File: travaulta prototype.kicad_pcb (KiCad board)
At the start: 4 copper layers, 209.7 x 76.4 mm, 106 parts, among them SW1 EC_SW, SW10 EC_SW, SW11 EC_SW, SW12 EC_SW, SW13 EC_SW, SW14 EC_SW, SW15 EC_SW, SW16 EC_SW, SW17 EC_SW, SW18 EC_SW, SW19 EC_SW, SW2 EC_SW, SW20 EC_SW, SW21 EC_SW, SW22 EC_SW, SW23 EC_SW, SW24 EC_SW, SW25 EC_SW, SW26 EC_SW, SW27 EC_SW, SW28 EC_SW, SW29 EC_SW, SW3 EC_SW, SW30 EC_SW, SW31 EC_SW, SW32 EC_SW, SW33 EC_SW, SW34 EC_SW, SW35 EC_SW, SW36 EC_SW, SW37 EC_SW, SW38 BOOT0, SW4 EC_SW, SW5 EC_SW, SW6 EC_SW, SW7 EC_SW, SW8 EC_SW, SW9 EC_SW, U1 STM32F401CBUx, U2 XC6206PxxxMR, U3 74HC4051, U4 74HC4051, U5 OPA350, Y1 8 MHz

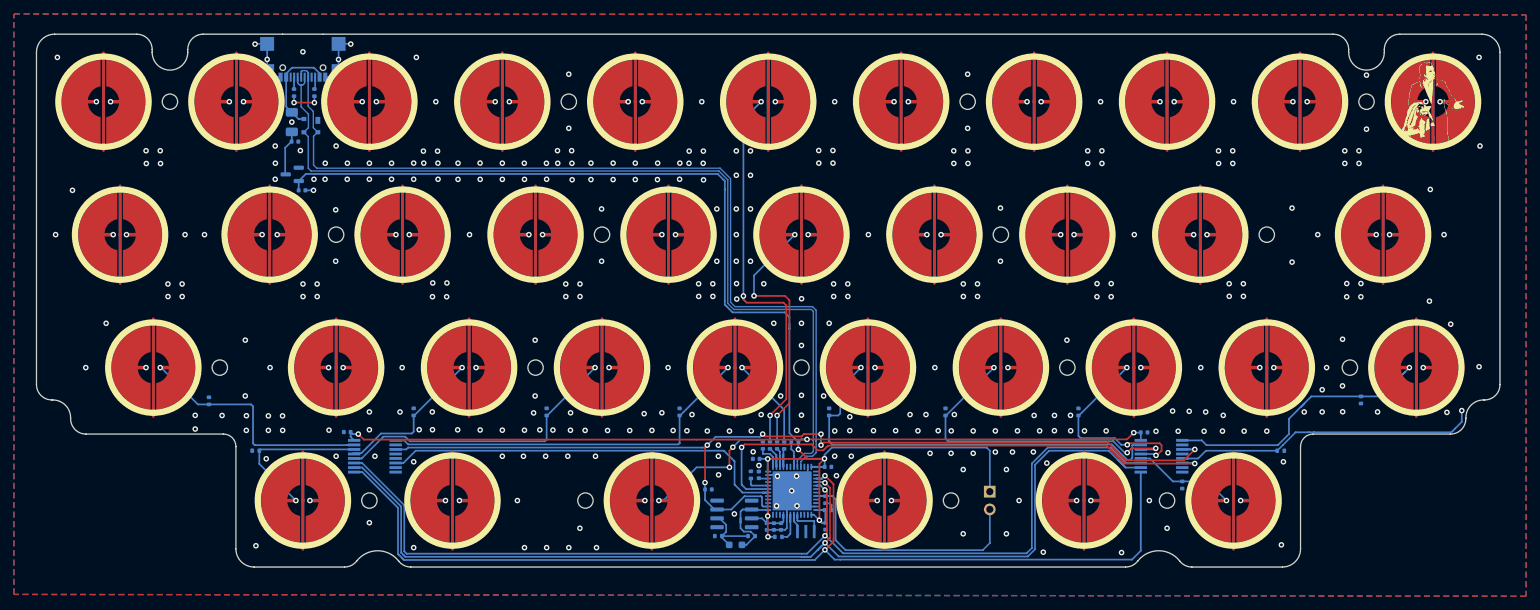
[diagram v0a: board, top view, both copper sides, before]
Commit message: pcb clean up, fresh gerbers
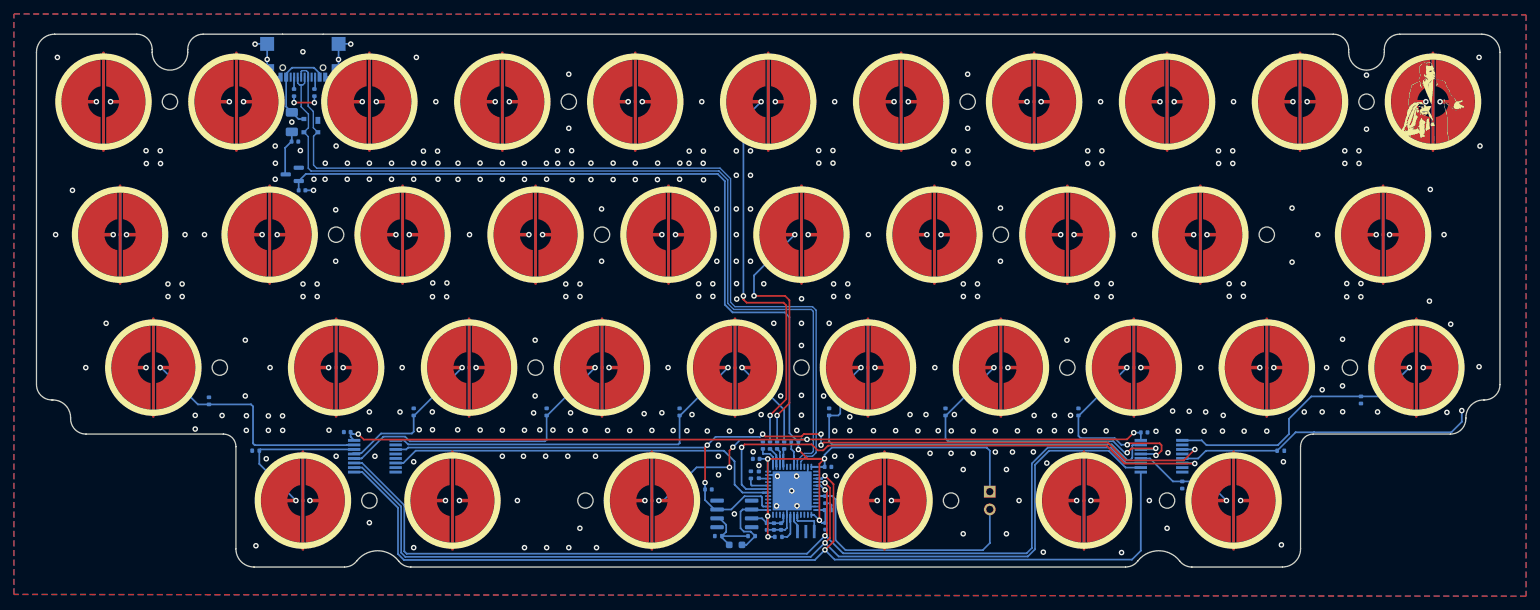
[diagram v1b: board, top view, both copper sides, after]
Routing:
- net COL9: track 91.0 -> 85.8 mm
- net AMUX_SEL_1: track 153.5 -> 149.5 mm
- net VBAT: track 319.6 -> 318.1 mm
- net APLEX_OUT_PIN_0: track 141.9 -> 140.6 mm
- net ADC: track 12.5 -> 11.5 mm
- net ROW3: track 222.5 -> 221.9 mm
